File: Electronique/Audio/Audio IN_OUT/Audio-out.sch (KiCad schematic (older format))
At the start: 49 parts, among them Q3001 BSS123, U3001 MC33172, U3002 MF10, U3003 TDA2003

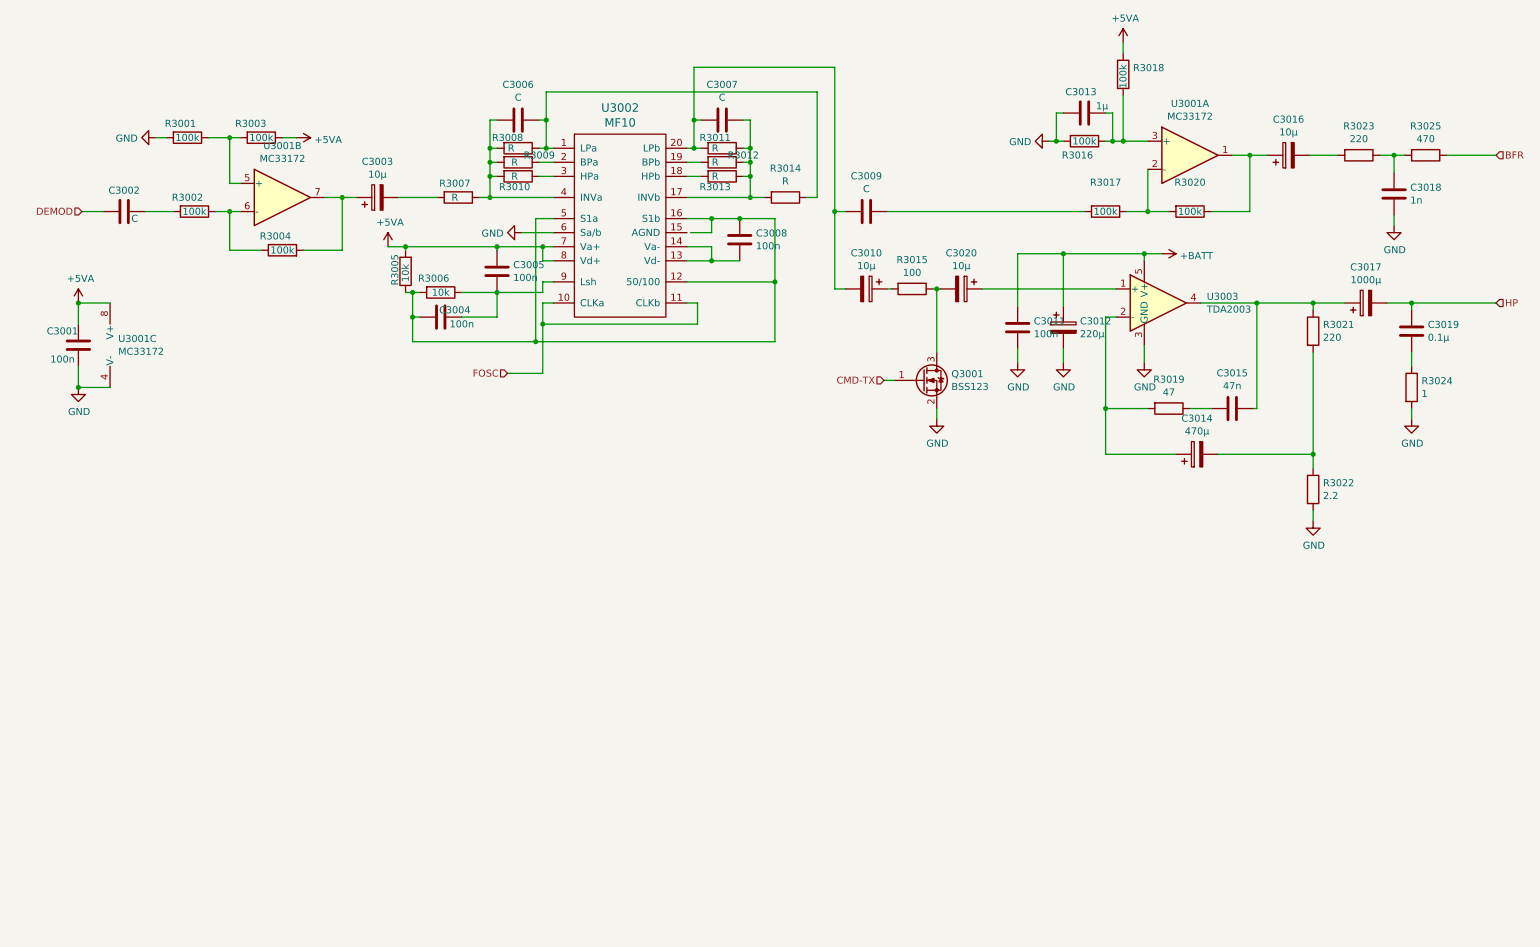
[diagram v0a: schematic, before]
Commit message: PIC32MZ_EF_100
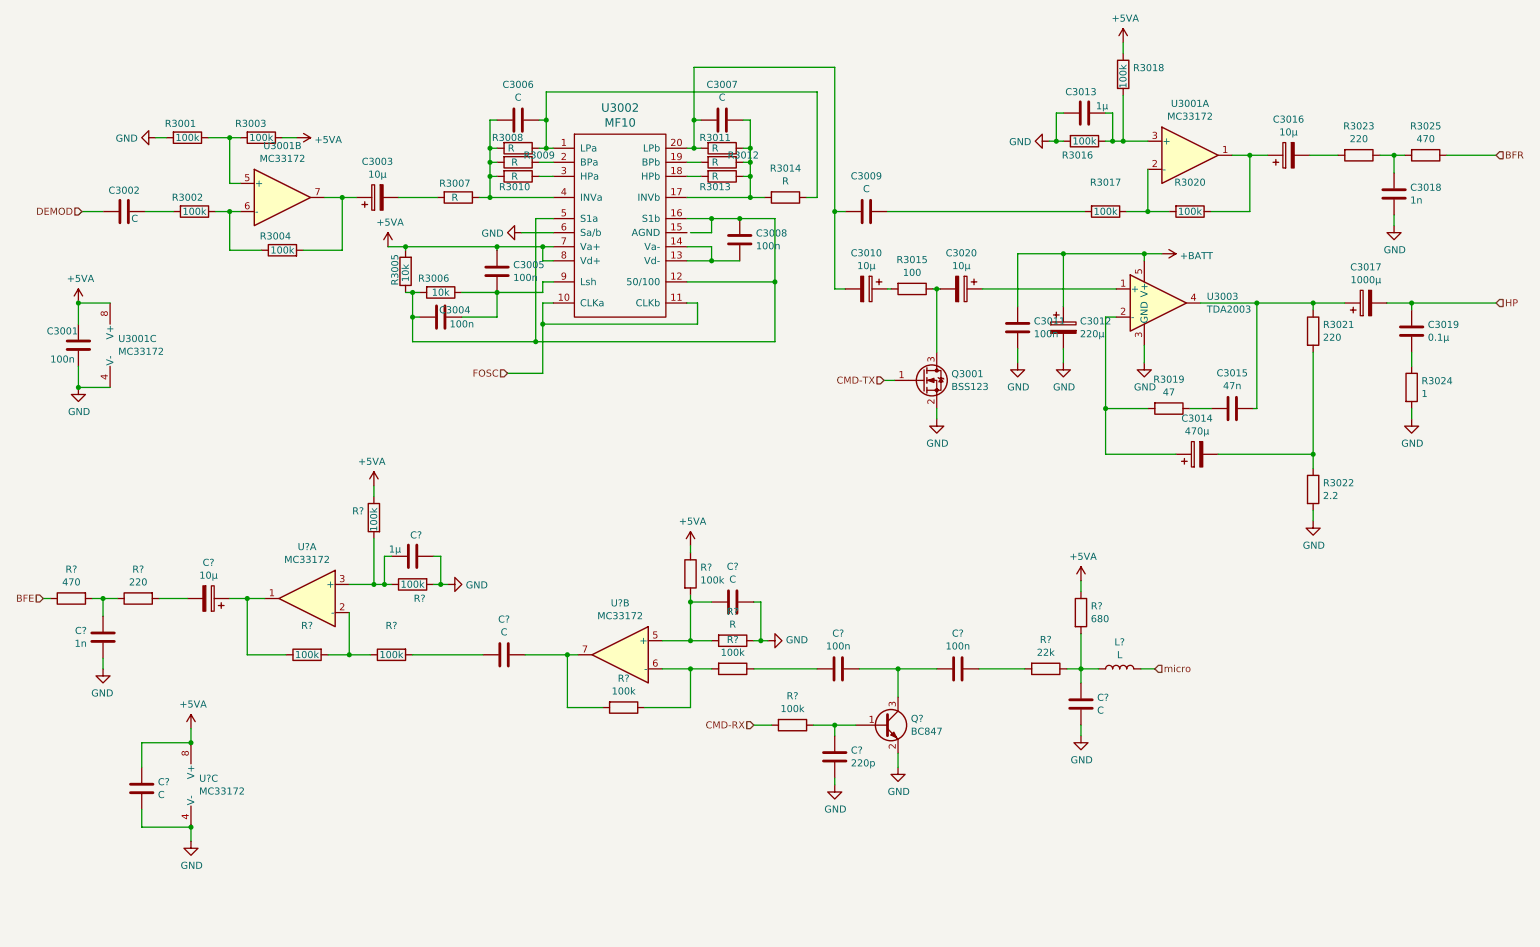
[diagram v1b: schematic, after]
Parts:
- added C?: C, Capacitor_SMD:C_0603_1608Metric, symbol Device:C
- added C?: 10µ, Capacitor_Tantalum_SMD:CP_EIA-3216-18_Kemet-A, symbol Device:CP
- added C?: 1n, Capacitor_SMD:C_0603_1608Metric, symbol Device:C
- added C?: 1µ, Capacitor_SMD:C_1210_3225Metric, symbol Device:C
- added C? (x3): C, symbol Device:C
- added C? (x2): 100n, symbol Device:C
- added C?: 220p, symbol Device:C
- added L?: L, symbol Device:L
- added Q?: BC847, Package_TO_SOT_SMD:SOT-23, symbol Transistor_BJT:BC847
- added R? (x4): 100k, Resistor_SMD:R_0603_1608Metric, symbol Device:R
- added R?: 220, Resistor_SMD:R_0603_1608Metric, symbol Device:R
- added R?: 470, Resistor_SMD:R_0603_1608Metric, symbol Device:R
- added R? (x4): 100k, symbol Device:R
- added R?: R, symbol Device:R
- added R?: 680, symbol Device:R
- added R?: 22k, symbol Device:R
- added U? (x3): MC33172, symbol Amplifier_Operational:MC33172
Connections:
- net +5VA: now also C?.1, R?.1, R?.1, R?.1, U?.8 (V+)
- net GND: now also C?.1, C?.2, C?.2, C?.2, C?.2, C?.2, Q?.2 (E), R?.1, R?.2, U?.4 (V-)
- new net: C?.1, R?.1, U?.1
- new net: R?.1, R?.2, U?.2 (-)
- new net: C?.1, R?.1, R?.2, U?.3 (+)
- new net: C?.1, R?.2
- new net: C?.2, R?.2, U?.7
- new net: C?.2, R?.2 (x2)
- new net: C?.1, R?.1, R?.2
- new net: C?.2, R?.2, R?.2, U?.5 (+)
- new net: R?.1, R?.2, U?.6 (-)
- new net: C?.2, R?.1
- new net: C?.1, L?.1, R?.1, R?.2
- new net: C?.1, C?.1, Q?.3 (C)
- new net: C?.1, Q?.1 (B), R?.1
- new net BFE: R?.1
- new net CMD-RX: R?.2
- new net micro: L?.2

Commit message: CONNECTOR BOARD V2.00
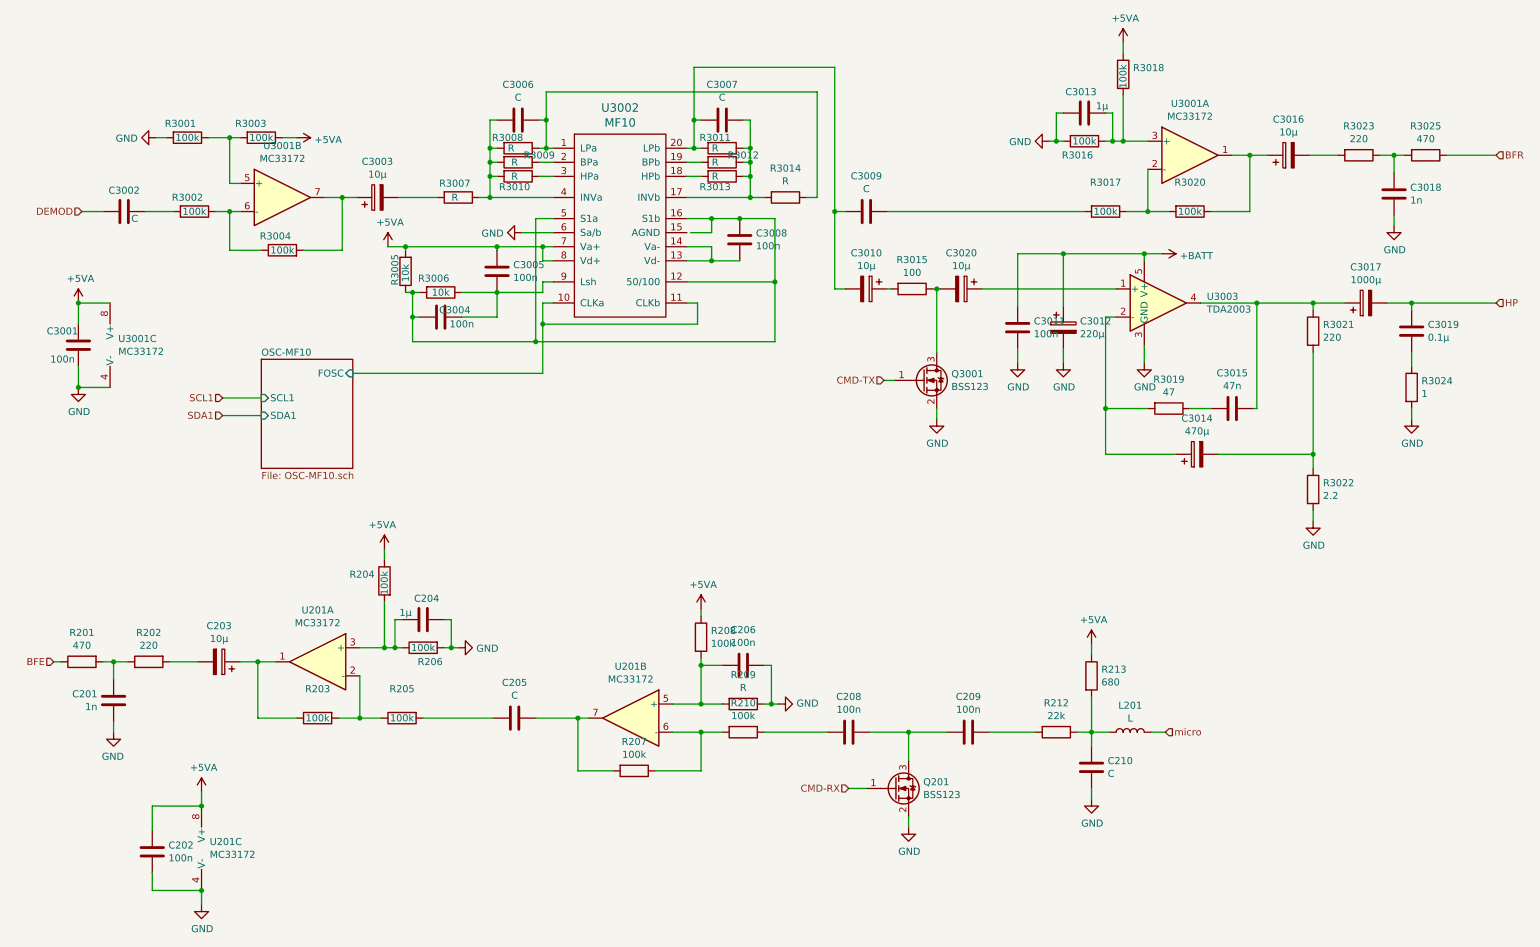
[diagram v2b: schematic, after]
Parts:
- removed C?: 220p, symbol Device:C
- removed Q?: BC847, Package_TO_SOT_SMD:SOT-23, symbol Transistor_BJT:BC847
- removed R?: 100k, symbol Device:R
- added Q201: BSS123, Package_TO_SOT_SMD:SOT-23, symbol Transistor_FET:BSS123
- C202, C206: renamed from C?; value C -> 100n; footprint (none) -> Capacitor_SMD:C_0603_1608Metric
- C204: renamed from C?; footprint Capacitor_SMD:C_1210_3225Metric -> Capacitor_SMD:C_0805_2012Metric
- C208, C209, C210: renamed from C?; footprint (none) -> Capacitor_SMD:C_0603_1608Metric
- L201: renamed from L?; footprint (none) -> Capacitor_SMD:C_1206_3216Metric
- R207, R208, R209, R210, R212, R213: renamed from R?; footprint (none) -> Resistor_SMD:R_0603_1608Metric
- U201: renamed from U?; footprint (none) -> Package_SO:SO-8_3.9x4.9mm_P1.27mm
- U3003: footprint CEN-PCB:TDA2003V -> Package_TO_SOT_THT:TO-220-5_P3.4x3.8mm_StaggerOdd_Lead7.13mm_TabDown
- gave numbers to parts that had none: 9
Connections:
- net CMD-RX: now also Q201.1 (G)
- net GND: now also Q201.2 (S)
- net at C208.1, C209.1: now also Q201.3 (D)
- net FOSC renamed OSC-MF10/FOSC
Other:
- moved on the sheet: C201, C202, C203, C204, C205, C206, C208, C209, C210, L201, R201, R202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
